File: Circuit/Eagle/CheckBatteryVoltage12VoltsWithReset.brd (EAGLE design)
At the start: 100.3 x 70 mm, 111 parts

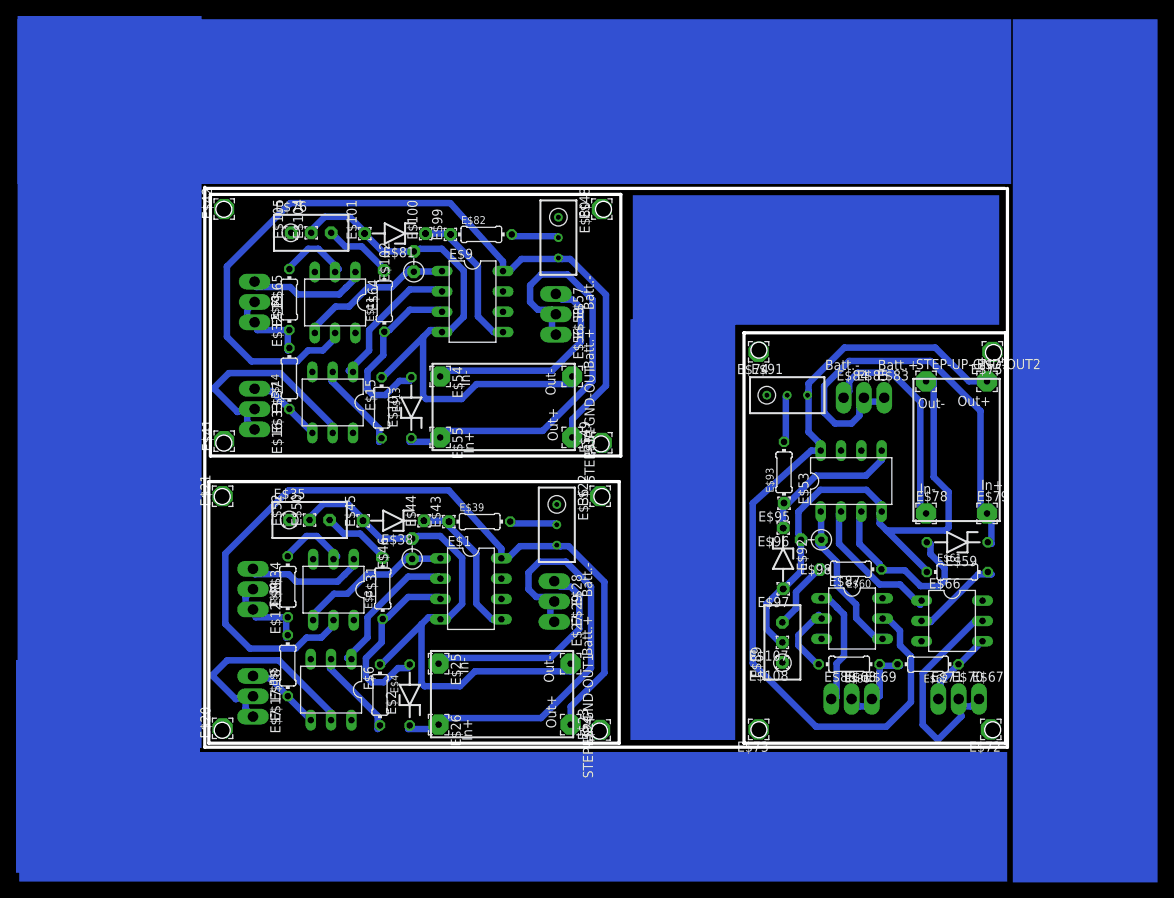
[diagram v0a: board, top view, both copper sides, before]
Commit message: .
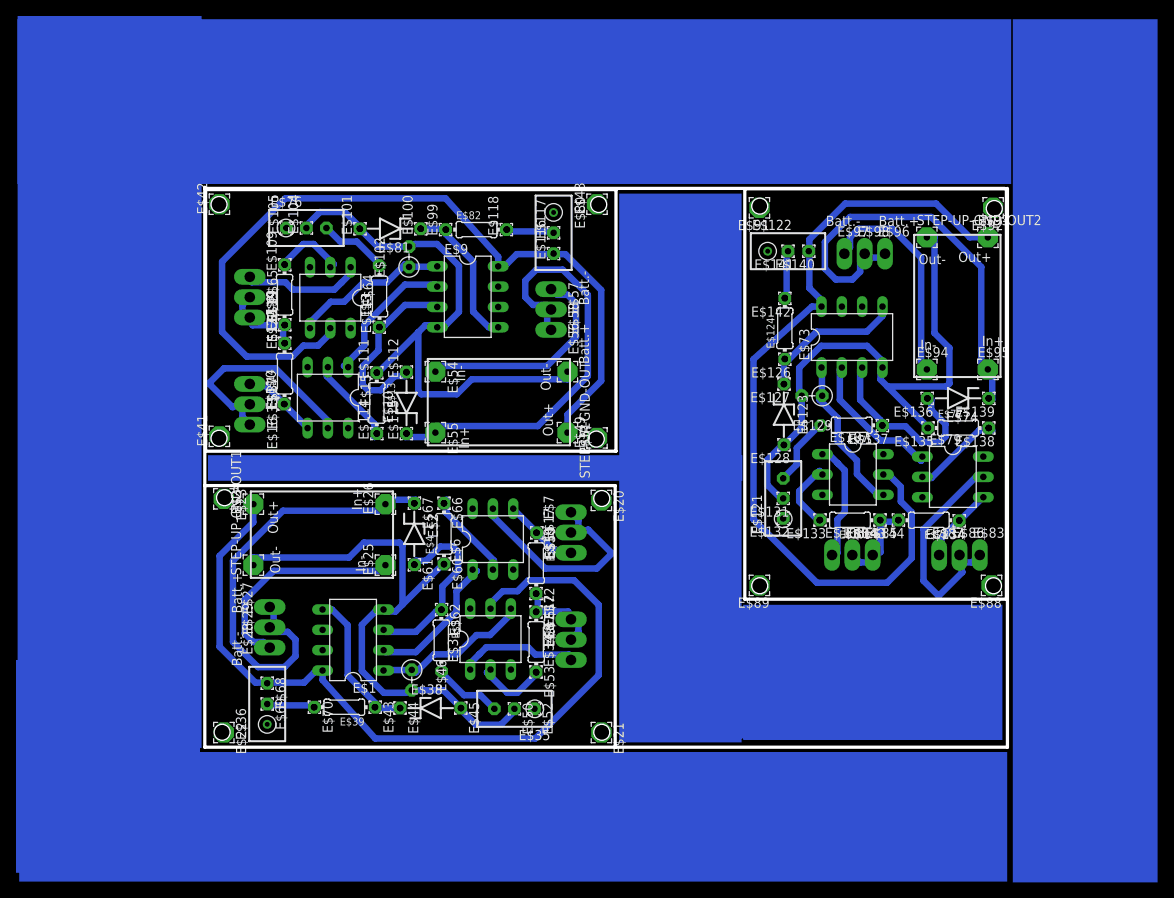
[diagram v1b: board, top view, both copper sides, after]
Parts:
- added E$109, E$110, E$111, E$112, E$113, E$114, E$115, E$116, E$117, E$118, E$119, E$120, E$125, E$126, E$127, E$128, E$130, E$131, E$132, E$133, E$134, E$135, E$136, E$137, E$138, E$139, E$140, E$141, E$142, E$143, E$144: (no value), wirepad:1,6/0,8
- added E$121: W203, rcl:RTRIM3296W
- added E$122: w501, rcl:RTRIM3296W
- added E$123: zener 4.3v, ref-packages-longpad:ZDIO-7.5
- added E$124: 100, eagle-ltspice:0204/7
- added E$129: (no value), discrete:RS-2,5
- E$106: value (none) -> 220; device wirepad:1,6/0,8 -> eagle-ltspice:0204/7
- E$107: value (none) -> Til113; device wirepad:1,6/0,8 -> ic-package:DIL06
- E$108, E$96, E$97: device wirepad:1,6/0,8 -> testpad:P1-13Y
- E$53: value Attiny85 -> (none); device 74xx-us:DIL08 -> wirepad:1,6/0,8
- E$59: value zener 10v -> (none); device ref-packages-longpad:ZDIO-7.5 -> wirepad:1,6/0,8
- E$60: value 680 -> (none); device eagle-ltspice:0204/7 -> wirepad:1,6/0,8
- E$61, E$62: value 220 -> (none); device eagle-ltspice:0204/7 -> wirepad:1,6/0,8
- E$66: value Til113 -> (none); device ic-package:DIL06 -> wirepad:1,6/0,8
- E$67, E$68, E$69, E$70, E$71: device testpad:P1-13Y -> wirepad:1,6/0,8
- E$72: device wirepad:2,54/0,8 -> wirepad:1,6/0,8
- E$73: value (none) -> Attiny85; device wirepad:2,54/0,8 -> 74xx-us:DIL08
- E$74: value (none) -> zener 10v; device wirepad:2,54/0,8 -> ref-packages-longpad:ZDIO-7.5
- E$75: value (none) -> 680; device wirepad:2,54/0,8 -> eagle-ltspice:0204/7
- E$77, E$78: value (none) -> 220; device wirepad:2,54/0,8 -> eagle-ltspice:0204/7
- E$79: value (none) -> Til113; device wirepad:2,54/0,8 -> ic-package:DIL06
- E$86: value 220 -> (none); device eagle-ltspice:0204/7 -> testpad:P1-13Y
- E$87: value Til113 -> (none); device ic-package:DIL06 -> testpad:P1-13Y
- E$88: device testpad:P1-13Y -> wirepad:2,54/0,8
- E$89: value W203 -> (none); device rcl:RTRIM3296W -> wirepad:2,54/0,8
- E$91: value w501 -> (none); device rcl:RTRIM3296W -> wirepad:2,54/0,8
- E$92: value zener 4.3v -> (none); device ref-packages-longpad:ZDIO-7.5 -> wirepad:2,54/0,8
- E$93: value 100 -> (none); device eagle-ltspice:0204/7 -> wirepad:2,54/0,8
- E$94, E$95: device wirepad:1,6/0,8 -> wirepad:2,54/0,8
- E$98: device discrete:RS-2,5 -> testpad:P1-13Y
- moved E$70 80.5 mm to (13.7, 5.00), turned to 270 degrees
- moved E$69 75.6 mm to (7.80, 5.40), turned to 270 degrees
- moved E$67 74.7 mm to (26.2, 30.5), turned to 270 degrees
- moved E$68 73.1 mm to (7.80, 8.00), turned to 270 degrees
- moved E$61 67.9 mm to (26.2, 22.8), turned to 270 degrees
- moved E$66 65.2 mm to (29.9, 30.5)
- moved E$62 61.2 mm to (29.6, 17.2), turned to 270 degrees
- moved E$72 59.3 mm to (41.4, 19.2), turned to 270 degrees
- moved E$21 55.8 mm to (49.6, 1.83), turned to 270 degrees
- moved E$22 55.6 mm to (2.38, 1.83), turned to 270 degrees
- moved E$20 55.3 mm to (49.6, 30.8), turned to 270 degrees
- moved E$23 55.2 mm to (2.38, 31.0), turned to 270 degrees
- moved E$59 52.6 mm to (41.5, 26.8), turned to 270 degrees
- moved E$71 51.5 mm to (41.4, 16.9), turned to 270 degrees
- moved E$92 51.1 mm to (98.5, 67.4), turned to 180 degrees
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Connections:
- net 5.1V-STEP-UP2: now also E$107.5, E$122.3, E$73.8, E$93.1; no longer E$53.8, E$77.1, E$87.5, E$91.3
- net IN-12V-BATTERY2: now also E$74.C, E$95.1, E$96.TP, E$98.TP; no longer E$59.C, E$79.1, E$83.TP, E$85.TP
- net IN-5V-FROM-NANO-SDCARD2: now also E$79.5, E$83.TP, E$86.TP; no longer E$66.5, E$67.TP, E$70.TP
- net IN-GND-BATTERY2: now also E$94.1, E$97.TP; no longer E$78.1, E$84.TP
- net IN-GND-NANO-SD-CARD2: now also E$106.1, E$78.2, E$84.TP, E$85.TP; no longer E$62.2, E$68.TP, E$69.TP, E$86.1
- net IN-TO-RESET-ATTINY2: now also E$107.1, E$108.TP; no longer E$87.1, E$88.TP
- net OUT-SERIAL-DATA2: now also E$78.1, E$79.4, E$87.TP; no longer E$62.1, E$66.4, E$71.TP
- net PHOTO-DIODE2: now also E$77.2, E$79.2; no longer E$61.2, E$66.2
- net S$10: now also E$122.2, E$124.2; no longer E$91.2, E$93.2
- net S$11: now also E$107.4, E$129.1, E$73.1; no longer E$53.1, E$87.4, E$98.1
- net S$8: now also E$106.2, E$107.2; no longer E$86.2, E$87.2
- net S$9: now also E$121.3, E$75.2; no longer E$60.2, E$89.3
- net STEP-UP-GND2: now also E$121.2, E$123.A, E$129.2, E$73.4, E$77.1; no longer E$53.4, E$61.1, E$89.2, E$92.A, E$98.2
- net TX-SERIAL-DATA2: now also E$73.2, E$79.1; no longer E$53.2, E$66.1
- net VZ-ANALOG-REFERENCE2: now also E$123.C, E$124.1, E$73.5; no longer E$53.5, E$92.C, E$93.1
- net VZ-BATTERY-LEVEL2: now also E$73.3, E$74.A, E$75.1; no longer E$53.3, E$59.A, E$60.1
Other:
- outline, holes or cut-outs redrawn
